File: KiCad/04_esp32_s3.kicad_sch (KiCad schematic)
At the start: 32 parts, among them IC401 ESP32-S3-WROOM-1-N16R8, J401 TF-01A, Q401 SS8050, Q402 SS8050

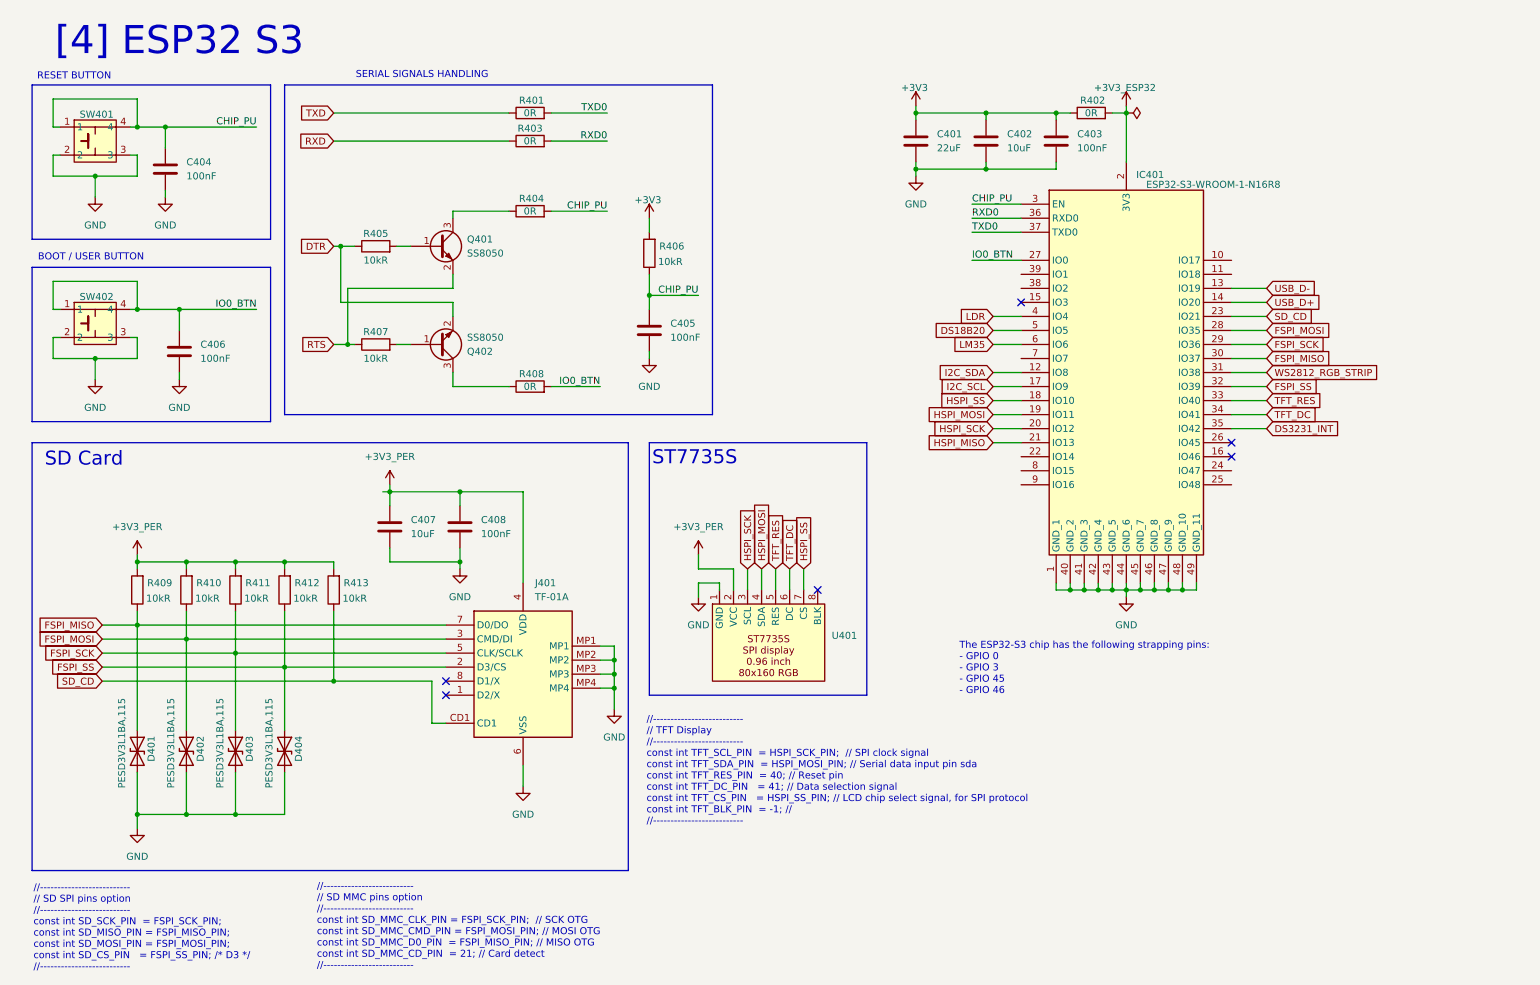
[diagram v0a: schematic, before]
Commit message: First scheme version
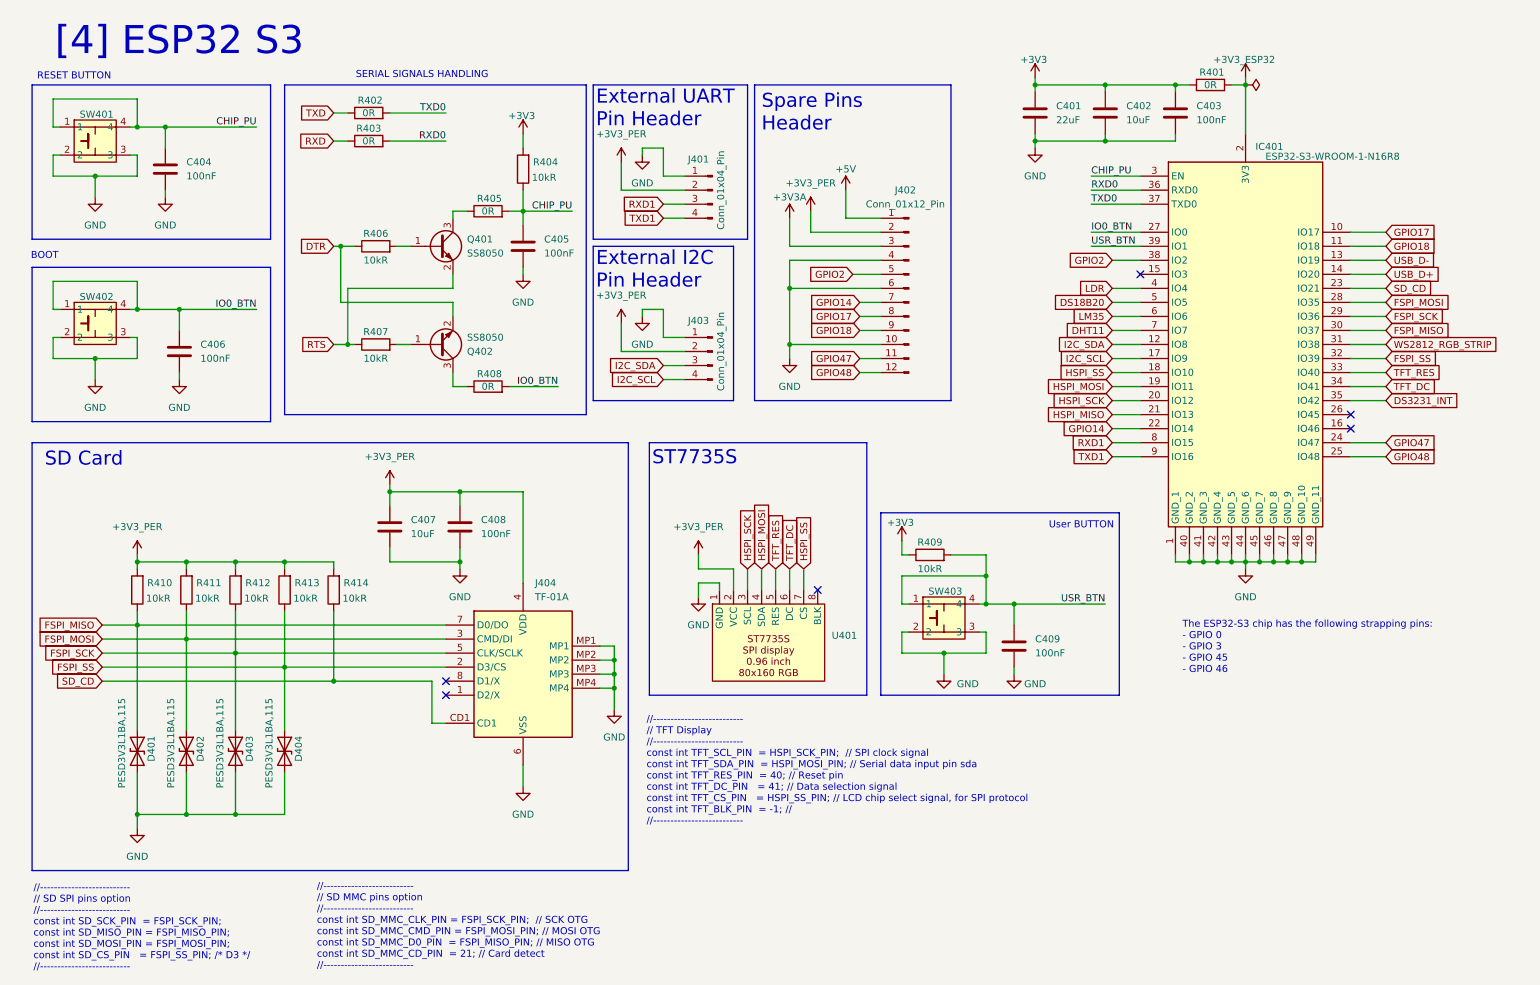
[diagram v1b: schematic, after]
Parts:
- added C409: 100nF, Capacitor_SMD:C_0603_1608Metric, symbol Device:C
- added J401, J403: Conn_01x04_Pin, Connector_PinHeader_2.54mm:PinHeader_1x04_P2.54mm_Vertical, symbol Connector:Conn_01x04_Pin
- added J402: Conn_01x12_Pin, Connector_PinHeader_2.54mm:PinHeader_1x12_P2.54mm_Vertical, symbol Connector:Conn_01x12_Pin
- added R409: 10kR, Resistor_SMD:R_0805_2012Metric, symbol Device:R
- added SW403: ~, esp32_s3_weather_webserver:SW_PUSH_6mm_H5mm, symbol esp32_s3_weather_webserver:SW_PUSH_6mm_H5mm
- Q401, Q402: Manufacturer Jiangsu Changjing Electronics Technology Co., Ltd. -> (none); Manufacturer Part Number SS8050(RANGE:200-350) -> (none)
- renumbered J401 to J404, R402 to R401, R401 to R402, R406 to R404, R404 to R405, R405 to R406, R409 to R410, R410 to R411, R411 to R412, R412 to R413, R413 to R414
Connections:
- net +3V3: now also R409.1
- net +3V3_PER: now also J401.2 (Pin_2), J402.2 (Pin_2), J403.2 (Pin_2)
- net GND: now also C409.2, J401.1 (Pin_1), J402.10 (Pin_10), J402.4 (Pin_4), J402.6 (Pin_6), J403.1 (Pin_1), SW403.2, SW403.3
- net I2C_SCL: now also J403.4 (Pin_4)
- net I2C_SDA: now also J403.3 (Pin_3)
- net GPIO17: now reaches IC401.10 (IO17)
- net GPIO17: now also J402.8 (Pin_8)
- net GPIO18: now reaches IC401.11 (IO18)
- net GPIO18: now also J402.9 (Pin_9)
- net GPIO14: now reaches IC401.22 (IO14)
- net GPIO14: now also J402.7 (Pin_7)
- net GPIO47: now reaches IC401.24 (IO47)
- net GPIO47: now also J402.11 (Pin_11)
- net GPIO48: now reaches IC401.25 (IO48)
- net GPIO48: now also J402.12 (Pin_12)
- net GPIO2: now reaches IC401.38 (IO2)
- net GPIO2: now also J402.5 (Pin_5)
- net USR_BTN: now reaches IC401.39 (IO1)
- net USR_BTN: now also C409.1, R409.2, SW403.1, SW403.4
- net DHT11: now reaches IC401.7 (IO7)
- net RXD1: now reaches IC401.8 (IO15)
- net RXD1: now also J401.3 (Pin_3)
- net TXD1: now reaches IC401.9 (IO16)
- net TXD1: now also J401.4 (Pin_4)
- new net +3V3A: J402.3 (Pin_3)
- new net +5V: J402.1 (Pin_1)
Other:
- note added: "BOOT"
- note added: "External I2C Pin Header"
- note added: "External UART Pin Header"
- note added: "Spare Pins Header"
- note added: "User BUTTON"
- note removed: "BOOT / USER BUTTON"
- moved on the sheet: C401, C402, C403, C405, IC401, R401, R402, R403, R404, R405, R408

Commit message: Firmware refactoring. Beginning
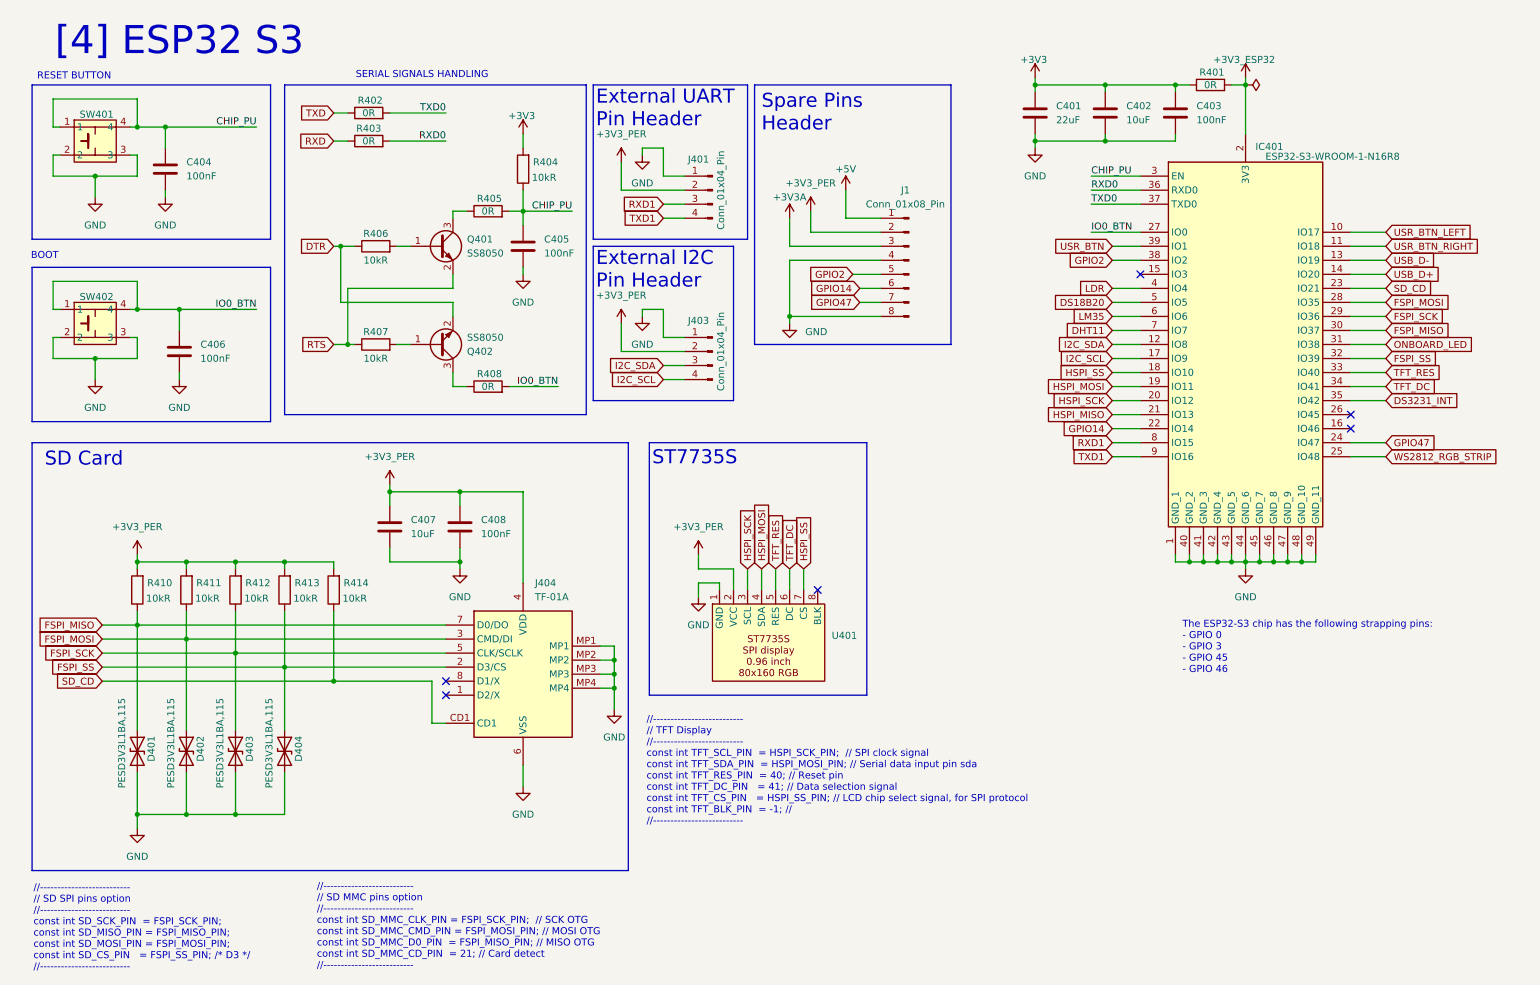
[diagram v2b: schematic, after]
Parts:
- removed C409: 100nF, Capacitor_SMD:C_0603_1608Metric, symbol Device:C
- removed J402: Conn_01x12_Pin, Connector_PinHeader_2.54mm:PinHeader_1x12_P2.54mm_Vertical, symbol Connector:Conn_01x12_Pin
- removed R409: 10kR, Resistor_SMD:R_0805_2012Metric, symbol Device:R
- removed SW403: ~, esp32_s3_weather_webserver:SW_PUSH_6mm_H5mm, symbol esp32_s3_weather_webserver:SW_PUSH_6mm_H5mm
- added J1: Conn_01x08_Pin, symbol Connector:Conn_01x08_Pin
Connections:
- net GPIO48 is gone; now on net WS2812_RGB_STRIP: IC401.25 (IO48)
- net +3V3A: now also J1.3 (Pin_3)
- net +3V3_PER: now also J1.2 (Pin_2)
- net +5V: now also J1.1 (Pin_1)
- net GND: now also J1.4 (Pin_4), J1.8 (Pin_8)
- net GPIO14: now also J1.6 (Pin_6)
- net GPIO2: now also J1.5 (Pin_5)
- net GPIO47: now also J1.7 (Pin_7)
- net WS2812_RGB_STRIP: no longer IC401.31 (IO38)
- net GPIO17 renamed USR_BTN_LEFT
- net GPIO18 renamed USR_BTN_RIGHT
- new net ONBOARD_LED: IC401.31 (IO38)
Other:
- note removed: "User BUTTON"
